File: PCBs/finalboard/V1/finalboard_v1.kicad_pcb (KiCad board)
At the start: 2 copper layers, 45 parts, among them J1 Conn_01x02_Socket, J10 Conn_01x01, J11 Conn_01x01, J12 Conn_01x01, J13 Conn_01x02_Socket, J2 Conn_01x02_Socket, J3 Conn_01x02_Socket, J4 Conn_01x02_Socket, J5 Conn_01x02_Socket, J6 USB_Conn, J7 Conn_01x02_Socket, J8 Conn_01x02_Socket, J9 Conn_01x01, U1 LD1117S33TR_SOT223, U2 STM32F405RGTx, U4 LSM6DSL, Y1 MAX7375AXR805

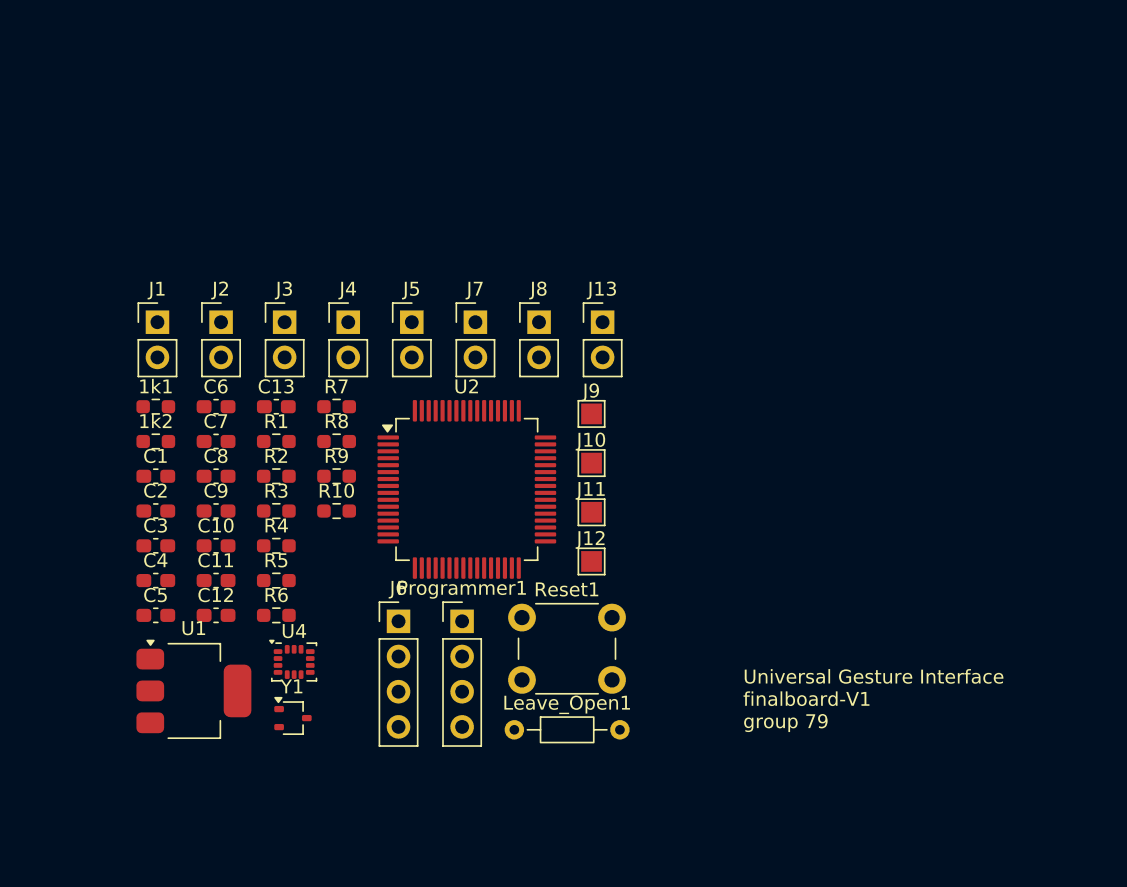
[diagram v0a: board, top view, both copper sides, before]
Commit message: Finalboard-V1 layout done (by kenobi)
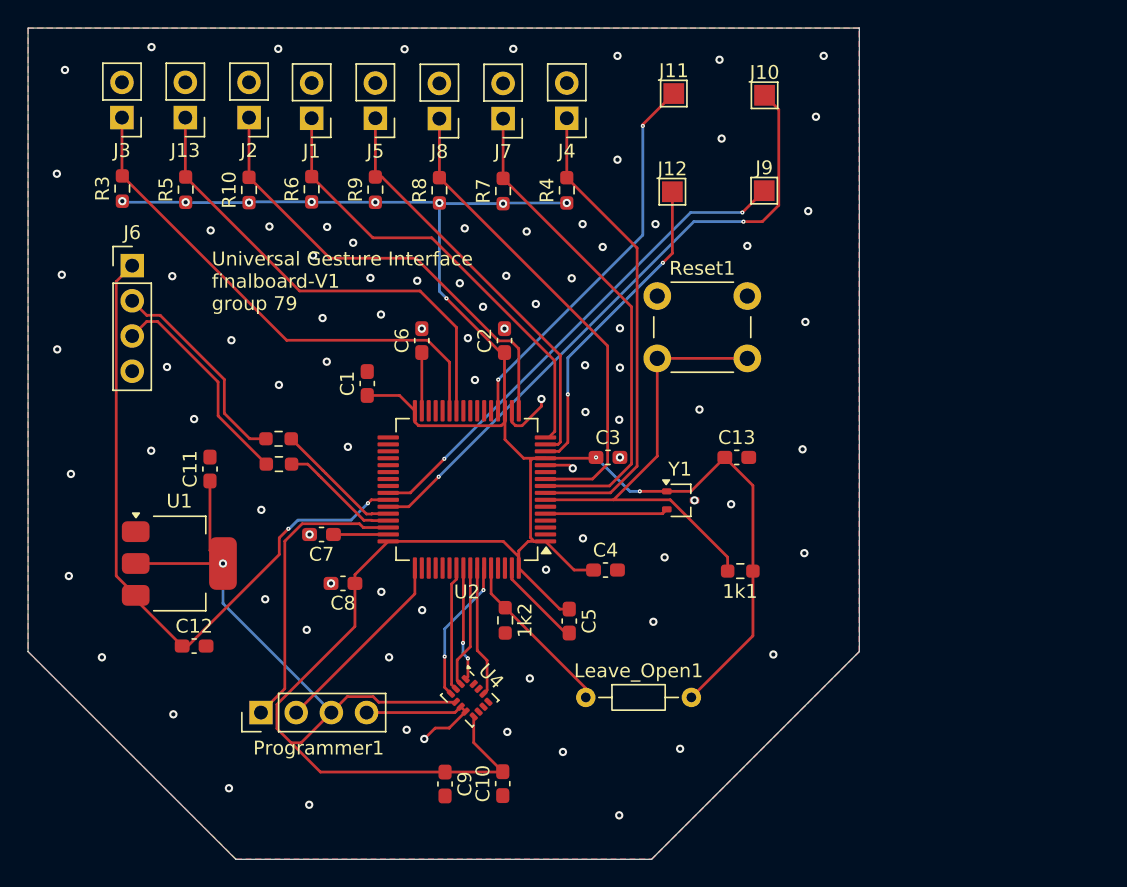
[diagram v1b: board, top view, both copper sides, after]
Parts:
- moved 1k1 43.8 mm to (181.4, 109.2), turned to 180 degrees
- moved J13 33.5 mm to (141.4, 76.5), turned to 180 degrees
- moved C13 33.4 mm to (181.2, 101.0)
- moved C3 33.3 mm to (171.9, 101.0)
- moved R4 33.1 mm to (168.9, 81.7), turned to 90 degrees
- moved C4 32.5 mm to (171.7, 109.1)
- moved Y1 32.1 mm to (177.1, 104.1)
- moved J6 32.1 mm to (137.5, 87.1)
- moved R6 30.9 mm to (150.5, 81.6), turned to 90 degrees
- moved J11 30.8 mm to (176.6, 74.7)
- moved C5 29.8 mm to (169.1, 112.8), turned to -90 degrees
- moved J10 29.3 mm to (183.2, 74.9)
- moved R5 29.0 mm to (141.4, 81.7), turned to 90 degrees
- moved 1k2 28.3 mm to (164.4, 112.8), turned to -90 degrees
- moved C2 28.0 mm to (164.4, 92.6), turned to 90 degrees
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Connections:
- net Net-(J6-Pin_2) renamed /USB-
- net Net-(J6-Pin_3) renamed /USB+
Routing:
- net VCC: track 0.00 -> 212.8 mm, vias 0 -> 12
- net /USB_VBUS_5V: track 0.00 -> 49.9 mm, vias 0 -> 2
- net /DEBUG_2: track 0.00 -> 45.6 mm, vias 0 -> 2
- net /ADC_FSR2: track 0.00 -> 36.9 mm
- net /DEBUG_1: track 0.00 -> 36.2 mm, vias 0 -> 2
- net /ADC_FSR4: track 0.00 -> 35.6 mm
- net /ADC_FSR5: track 0.00 -> 34.9 mm
- net /ADC_FSR3: track 0.00 -> 34.6 mm
- net /ADC_FSR1: track 0.00 -> 34.4 mm
- net Net-(U2-NRST): track 0.00 -> 33.9 mm
- net /ADC_FLEX3: track 0.00 -> 33.4 mm
- net /ADC_FLEX2: track 0.00 -> 33.2 mm
- net /ADC_FLEX1: track 0.00 -> 30.3 mm
- net /DEBUG_3: track 0.00 -> 28.2 mm, vias 0 -> 2
- net GND: track 0.00 -> 24.1 mm, vias 0 -> 87
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- added copper zone on B.Cu, net GND
- added copper zone on F.Cu, net GND
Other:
- board outline added: 60 x 60 mm
